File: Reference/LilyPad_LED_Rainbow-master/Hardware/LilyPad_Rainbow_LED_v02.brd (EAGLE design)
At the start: 38.6 x 12.7 mm, 37 parts

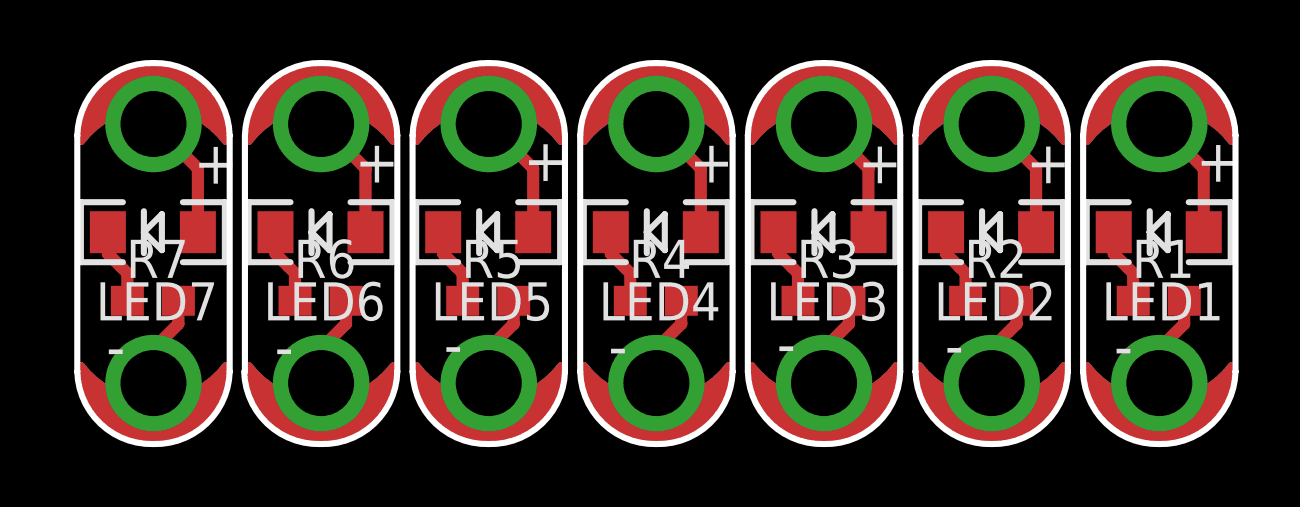
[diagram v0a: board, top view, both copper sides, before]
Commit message: v35 ready for initial review
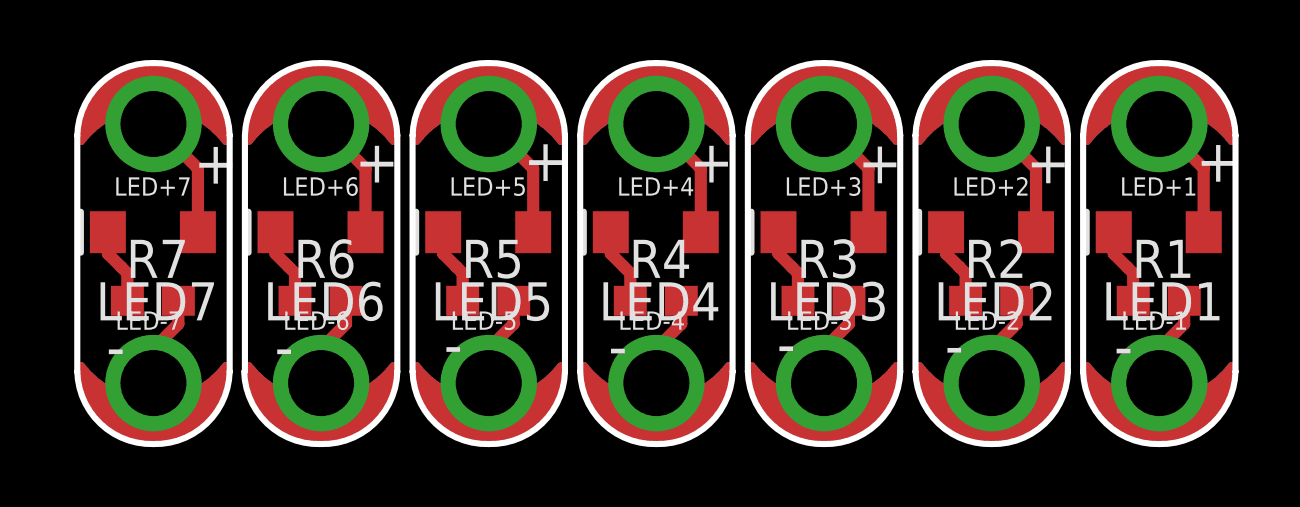
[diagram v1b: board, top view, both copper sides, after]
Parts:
- LED+1, LED+2, LED+3, LED+4, LED+5, LED+6, LED+7, LED-1, LED-2, LED-3, LED-4, LED-5, LED-6, LED-7: value SEWTAP6 -> SEWTAP_SMALL-2SIDE
- LED4: value YELLOW -> Yellow
- R1, R2, R3, R4, R5, R6, R7: device SparkFun-Resistors:0603-RES -> SparkFun-Resistors:0603
